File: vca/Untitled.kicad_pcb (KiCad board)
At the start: 2 copper layers, 74.2 x 82.8 mm, 116 parts, among them J1 AudioJack4, J10 V-, J11 V-, J12 V-, J13 V+, J14 V+, J15 V+, J2 Conn_01x10_Pin, J4 Conn_01x04_Pin, J6 V+, J7 V+, J8 V-, J9 V-, Q1 2N3906, Q2 2N3906, Q3 2N3906, Q4 2N3906, U1 LM13700, U10 LM13700, U11 TL072, U12 LM13700, U13 TL072, U2 TL074, U3 TL074, U4 LM7805_TO220, U5 TL072, U6 TL074, U7 TL074, U8 LM13700, U9 TL072

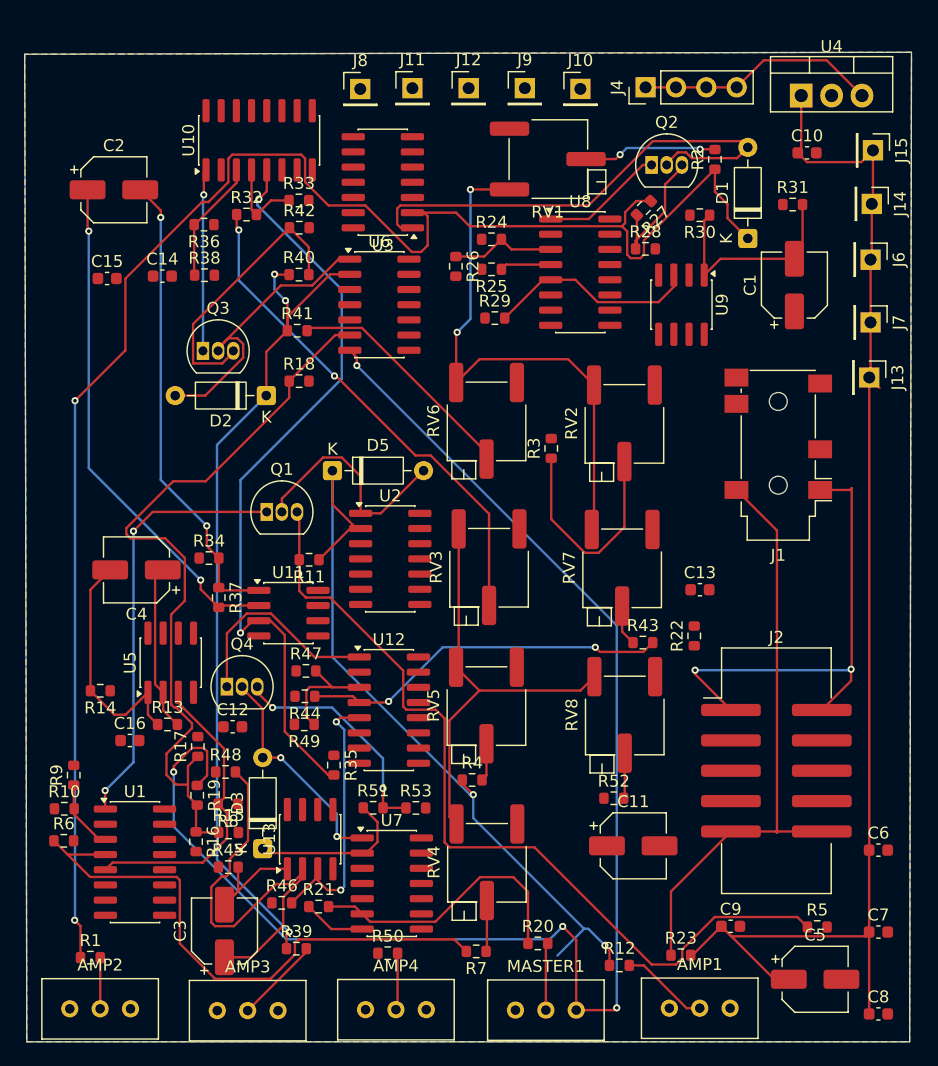
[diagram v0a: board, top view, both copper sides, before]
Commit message: finished the mod synth :D
(i keep on forgetting to commit :sob:)
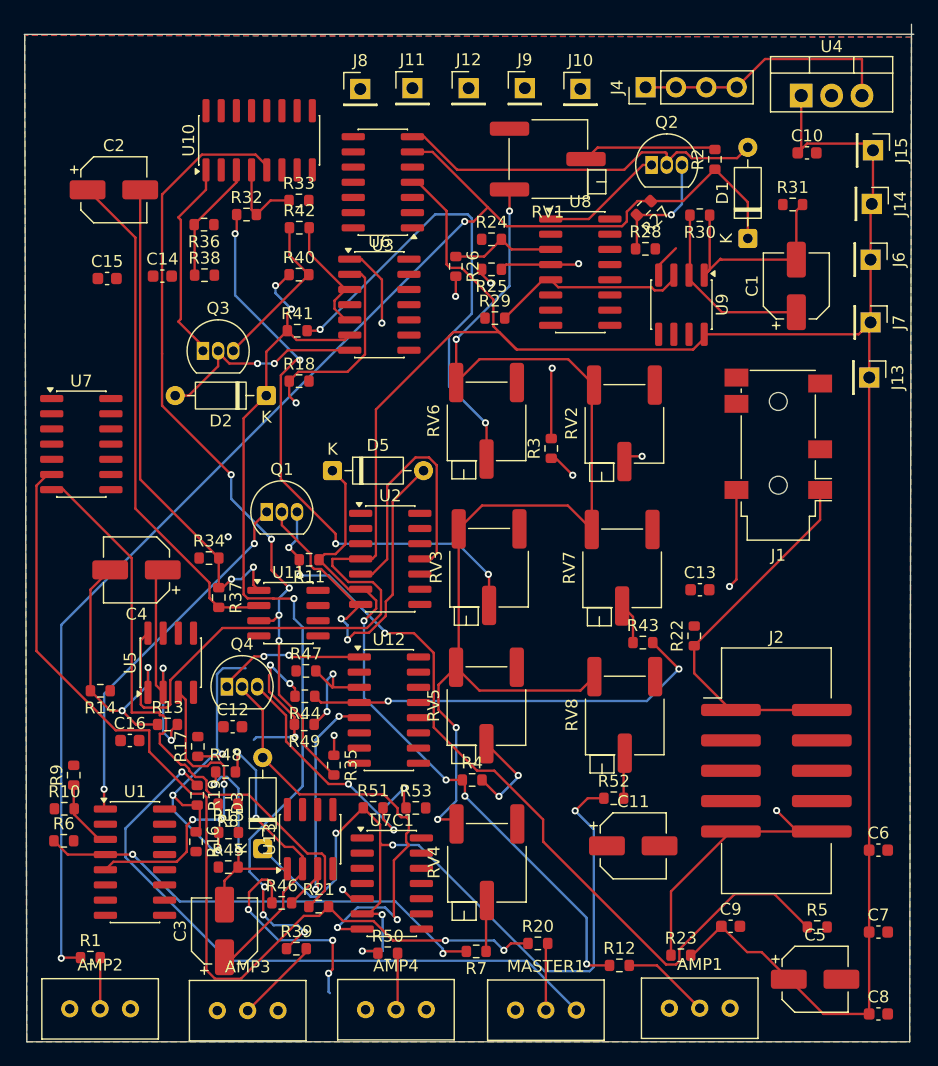
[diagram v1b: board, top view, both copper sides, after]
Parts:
- added G***: LOGO, LOGO, B.Cu at (131.5, 64.7)
- added U7: TL074, Package_SO:SOIC-14_3.9x8.7mm_P1.27mm, F.Cu at (90.7, 62.4)
- moved C1 0.17 mm to (150.5, 49.1)
- renumbered U7 to U7C1
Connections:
- AMP1 pad 1: unconnected-(AMP1-Pad1) -> GND
- AMP1 pad 3: GND -> unconnected-(AMP1-Pad3)
- AMP2 pad 1: unconnected-(AMP2-Pad1) -> GND
- AMP2 pad 3: GND -> unconnected-(AMP2-Pad3)
- AMP3 pad 1: unconnected-(AMP3-Pad1) -> GND
- AMP3 pad 3: GND -> unconnected-(AMP3-Pad3)
- AMP4 pad 1: unconnected-(AMP4-Pad1) -> GND
- AMP4 pad 3: GND -> unconnected-(AMP4-Pad3)
- R15 pad 1: Net-(U6B--) -> Net-(U6A--)
- R16 pad 1: Net-(U6B--) -> Net-(U6A--)
- R17 pad 1: Net-(U6B--) -> Net-(U6A--)
- R18 pad 1: Net-(U6B--) -> Net-(U6A--)
- R19 pad 2: Net-(U6B--) -> Net-(U6A--)
- U2 pad 1: Net-(D5-A) -> (no net)
- U2 pad 11: (no net) -> GND
- U2 pad 2: Net-(D5-K) -> (no net)
- U2 pad 3: GND -> (no net)
- U2 pad 4: (no net) -> +15V
- U2 pad 5: (no net) -> GND
- U2 pad 6: (no net) -> Net-(D5-K)
- U2 pad 7: (no net) -> Net-(D5-A)
- U3 pad 1: Net-(D1-A) -> (no net)
- U3 pad 11: (no net) -> GND
- U3 pad 2: Net-(D1-K) -> (no net)
- U3 pad 3: GND -> (no net)
- U3 pad 4: (no net) -> +15V
- U3 pad 5: (no net) -> GND
- U3 pad 6: (no net) -> Net-(D1-K)
- U3 pad 7: (no net) -> Net-(D1-A)
- U5 pad 4: (no net) -> GND
- U5 pad 8: (no net) -> +15V
- U6 pad 1: Net-(D2-A) -> Net-(MASTER1-Pad1)
- U6 pad 2: Net-(D2-K) -> Net-(U6A--)
- U6 pad 5: unconnected-(U6B-+-Pad5) -> GND
- U6 pad 6: Net-(U6B--) -> Net-(D2-K)
- U6 pad 7: Net-(MASTER1-Pad1) -> Net-(D2-A)
- U7C1 pad 1: Net-(D3-A) -> (no net)
- U7C1 pad 2: Net-(D3-K) -> (no net)
- U7C1 pad 3: GND -> (no net)
- U7C1 pad 6: Net-(U7B--) -> Net-(D3-K)
- U7C1 pad 7: unconnected-(R21-Pad1) -> Net-(D3-A)
- U9 pad 4: (no net) -> GND
- U9 pad 8: (no net) -> +15V
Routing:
- net GND: track 0.00 -> 134.8 mm, vias 0 -> 11
- net +15V: track 110.1 -> 221.5 mm
- net Net-(U6A--): track 0.00 -> 79.4 mm, vias 0 -> 4
- net Net-(U6B--): track 63.8 -> 0.00 mm
- net Net-(D3-K): track 13.5 -> 72.6 mm, vias 0 -> 5
- net Net-(U7B--): track 23.6 -> 81.9 mm, vias 0 -> 2
- net unconnected-(R21-Pad1): track 5.24 -> 50.7 mm
- net Net-(D1-K): track 140.6 -> 116.9 mm
- net Net-(R41-Pad2): track 20.0 -> 40.2 mm, vias 0 -> 2
- net Net-(D3-A): track 18.9 -> 38.7 mm
- net Net-(U8C--): track 4.29 -> 22.2 mm, vias 0 -> 2
- net Net-(MASTER1-Pad1): track 123.9 -> 107.0 mm, vias 4 -> 2
- net Net-(U9A--): track 0.00 -> 15.5 mm
- net VCC: track 82.3 -> 97.1 mm, vias 2 -> 4
- net Net-(D5-A): track 19.6 -> 32.6 mm, vias 0 -> 2
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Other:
- board size 74.2 x 82.8 mm -> 74.4 x 85.1 mm
- copper layers 2 -> 4
- board text added: "vca"
